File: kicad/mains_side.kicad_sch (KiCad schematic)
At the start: 40 parts, among them P1 Conn_WallPlug, Q1 Q_Photo_NPN, U2 B179

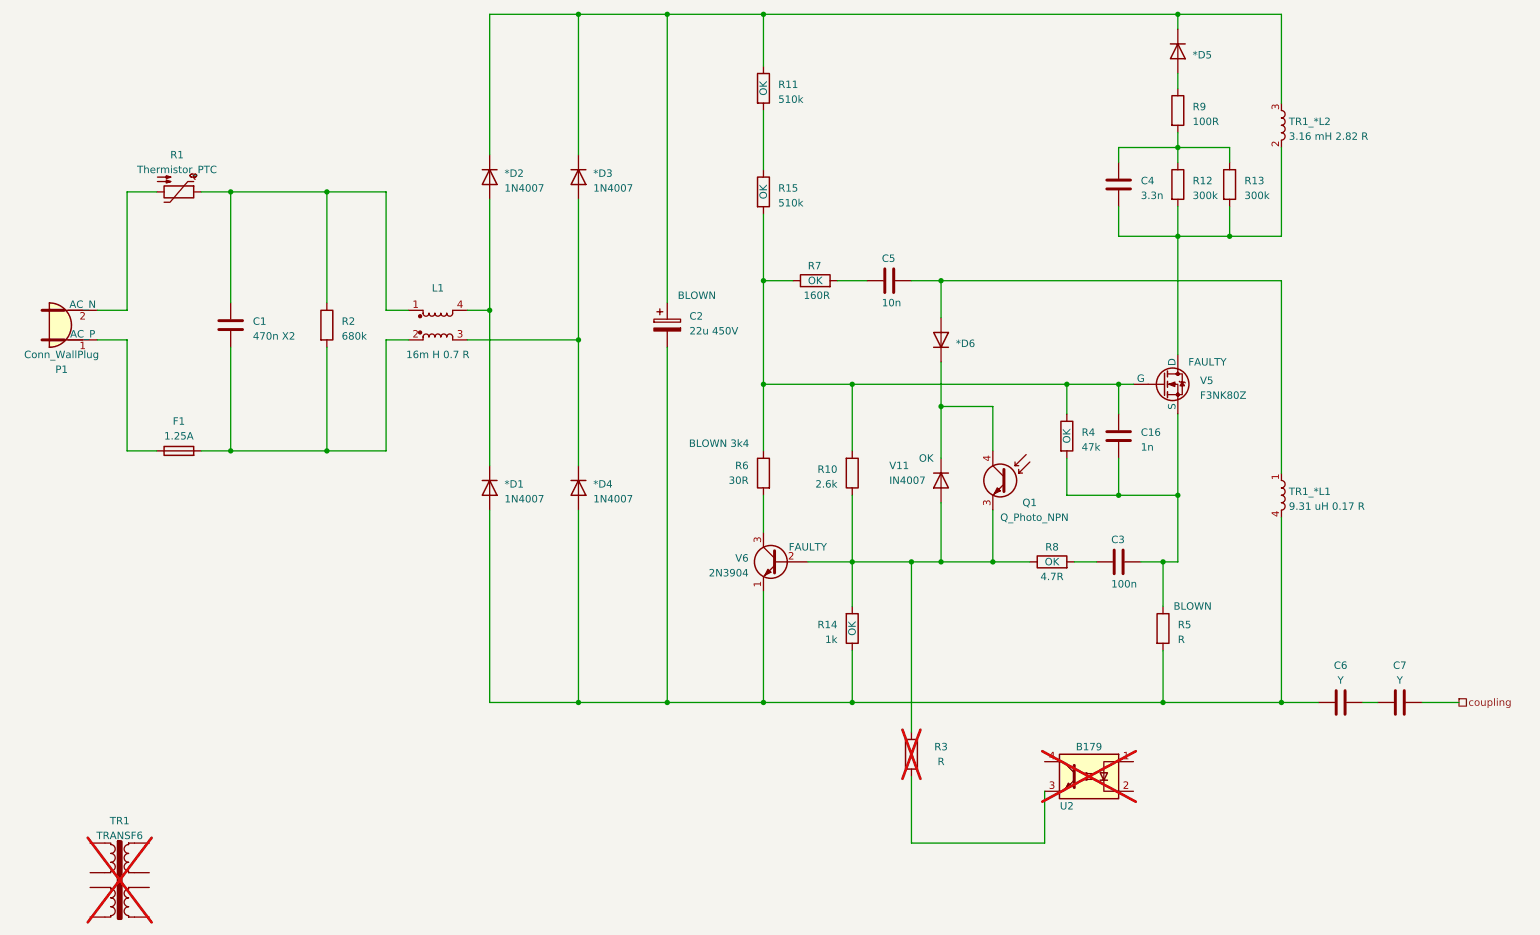
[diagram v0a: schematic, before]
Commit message: Update schematic
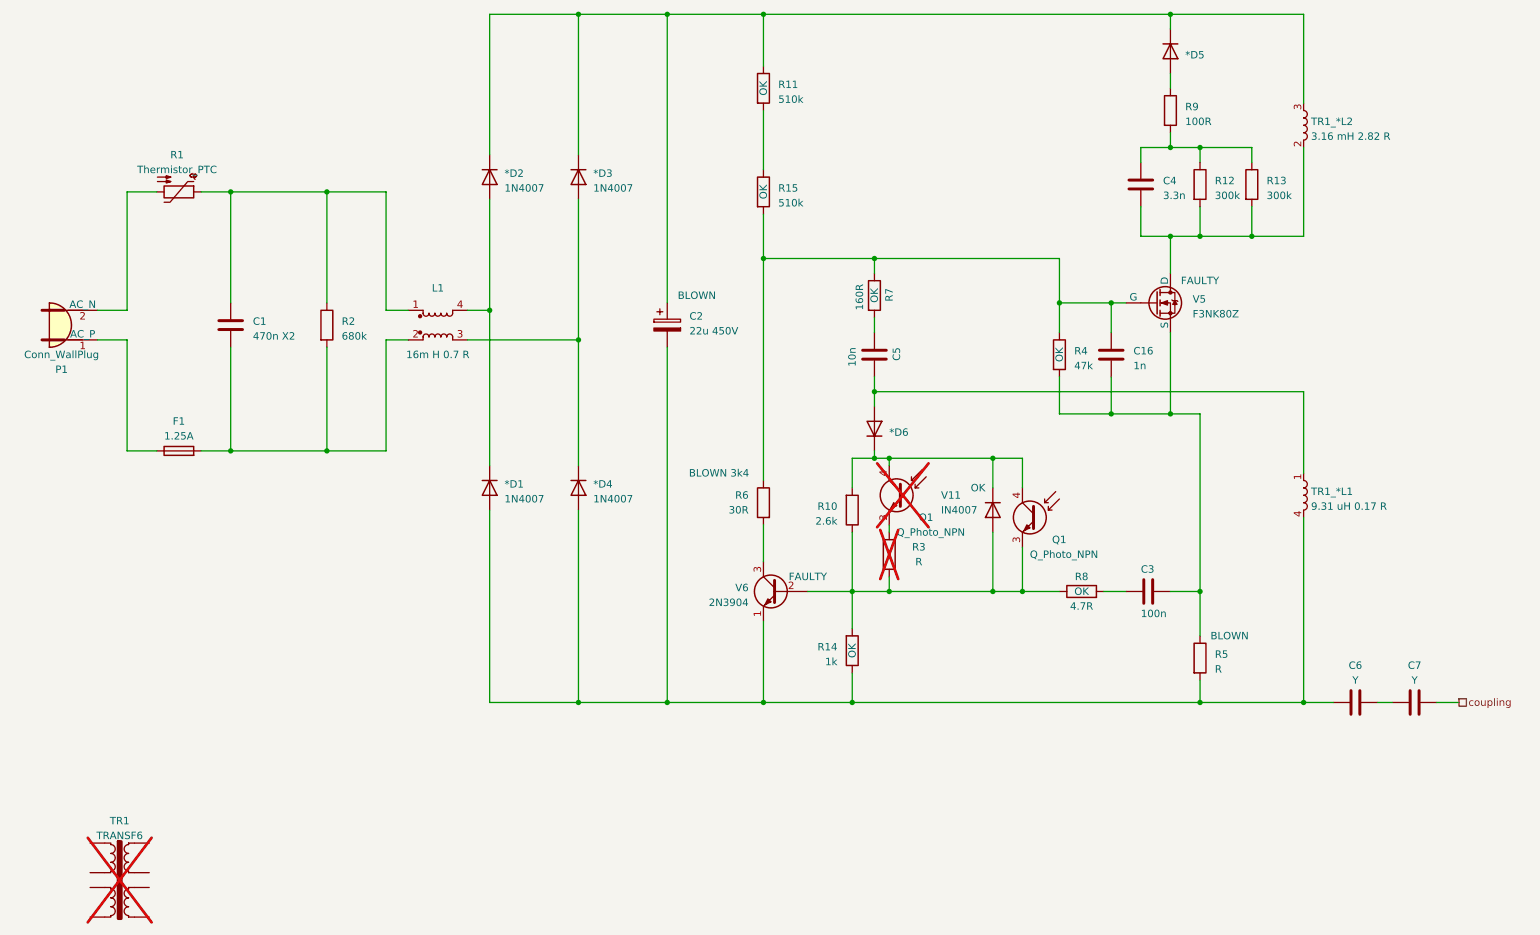
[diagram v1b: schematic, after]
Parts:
- removed U2: B179, Package_DIP:DIP-4_W7.62mm, symbol Isolator:EL817
- added Q1: Q_Photo_NPN, symbol Device:Q_Photo_NPN
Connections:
- net at Q1.3 (E), R10.1, R14.2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: now also R3.1; no longer R3.2
- net at C16.1, R15.2, R4.1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: no longer R10.2
- net at *D6.1 (K), Q1.4 (C), V11.1 (K): now also R10.2, Q1.4 (C)
- new net: Q1.3 (E), R3.2
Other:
- moved on the sheet: *D5, *D6, C16, C3, C4, C5, C6, C7, Q1, R10, R12, R13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
